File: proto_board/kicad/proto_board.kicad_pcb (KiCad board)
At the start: 2 copper layers, 80 x 50 mm, 3 parts, among them J1 pcie_98

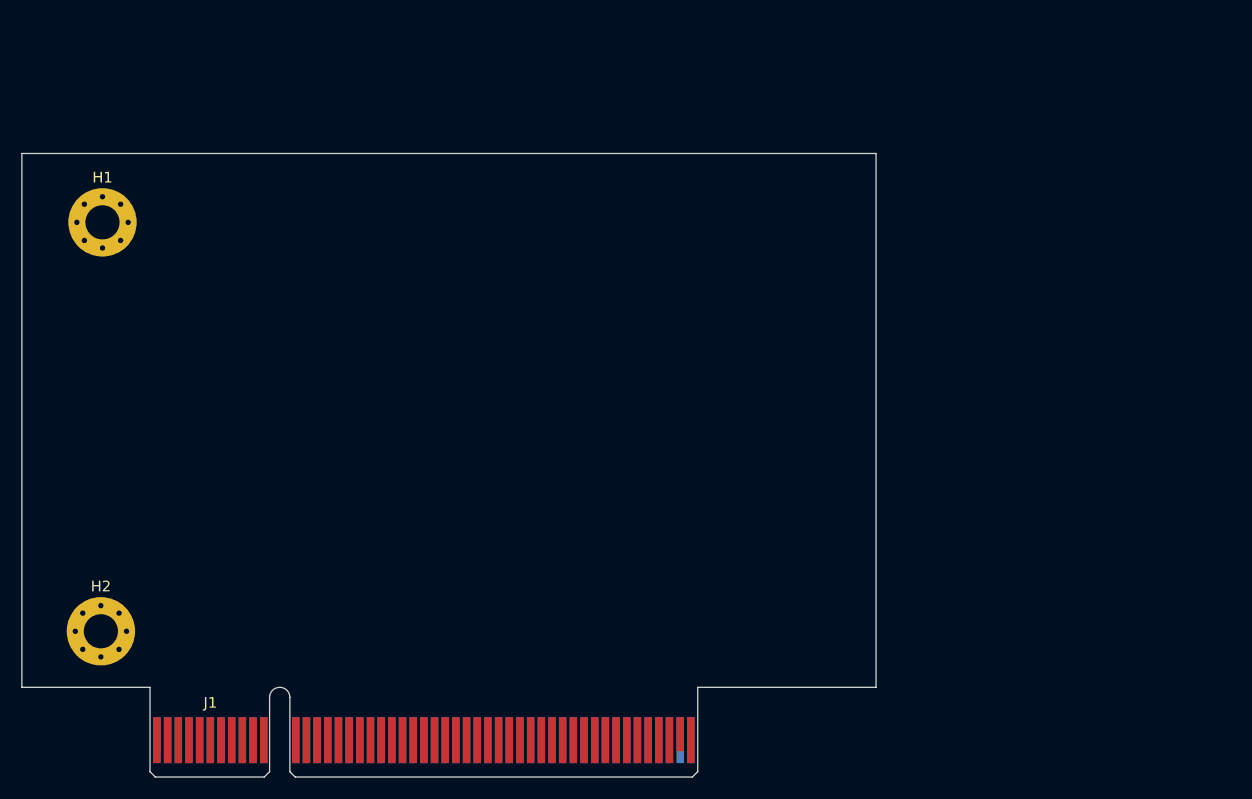
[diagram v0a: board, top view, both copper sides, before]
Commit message: Proto board work in progress.
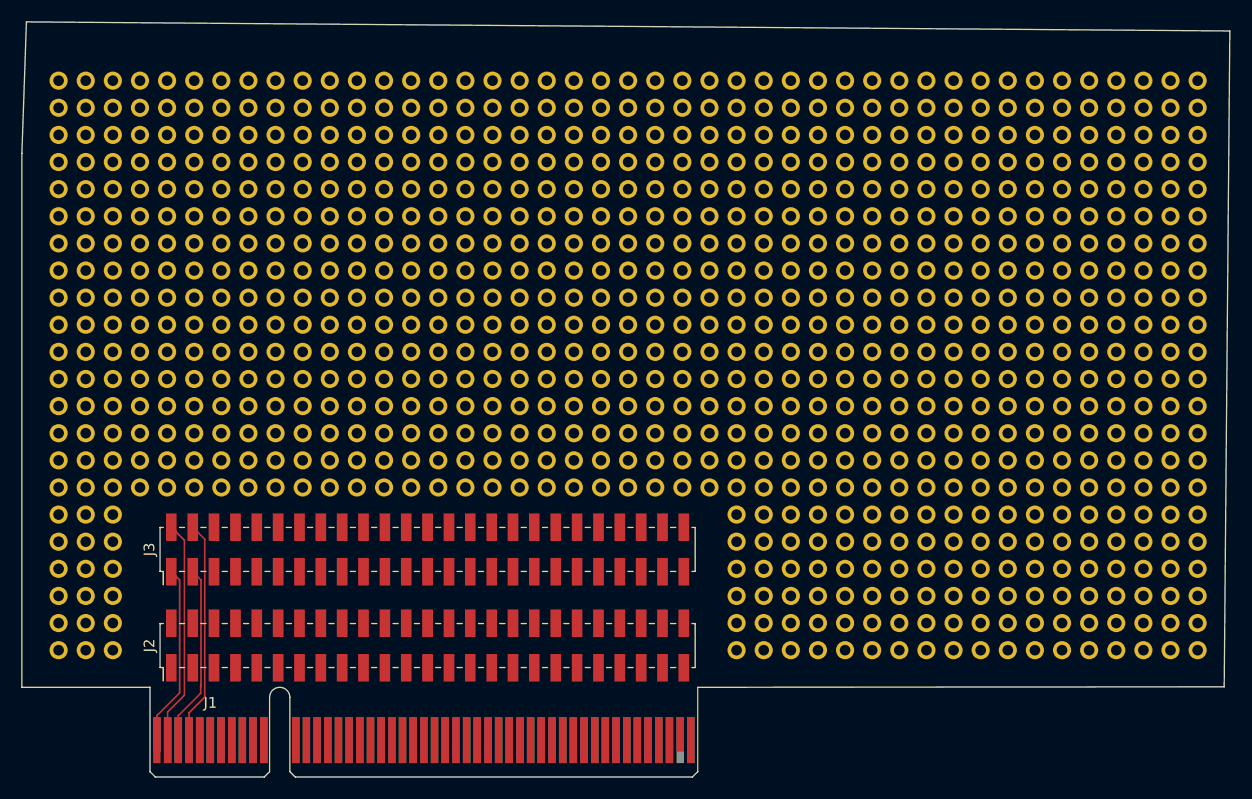
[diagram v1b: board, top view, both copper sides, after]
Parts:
- removed H1, H2: Bracket Hole, MountingHole:MountingHole_3.2mm_M3_Pad_Via
- added J2: Conn_02x25_Odd_Even, Connector_PinHeader_2.00mm:PinHeader_2x25_P2.00mm_Vertical_SMD, F.Cu at (126.0, 96.1)
- added J3: Conn_02x25_Odd_Even, Connector_PinHeader_2.00mm:PinHeader_2x25_P2.00mm_Vertical_SMD, F.Cu at (126.0, 87.1)
- added TP1: TestPoint, proto_board:pad, F.Cu at (147.3, 55.9)
- added TP1: TestPoint, proto_board:pad, F.Cu at (144.8, 55.9)
- added TP1: TestPoint, proto_board:pad, F.Cu at (162.6, 86.4)
- added TP1: TestPoint, proto_board:pad, F.Cu at (149.9, 78.7)
- added TP1: TestPoint, proto_board:pad, F.Cu at (94.0, 58.4)
- added TP1: TestPoint, proto_board:pad, F.Cu at (129.5, 53.3)
- added TP1: TestPoint, proto_board:pad, F.Cu at (175.3, 86.4)
- added TP1: TestPoint, proto_board:pad, F.Cu at (157.5, 83.8)
- added TP1: TestPoint, proto_board:pad, F.Cu at (177.8, 43.2)
- added TP1: TestPoint, proto_board:pad, F.Cu at (170.2, 78.7)
- added TP1: TestPoint, proto_board:pad, F.Cu at (144.8, 81.3)
- added TP1: TestPoint, proto_board:pad, F.Cu at (142.2, 50.8)
- added TP1: TestPoint, proto_board:pad, F.Cu at (190.5, 43.2)
- added TP1: TestPoint, proto_board:pad, F.Cu at (127.0, 43.2)
- added TP1: TestPoint, proto_board:pad, F.Cu at (134.6, 50.8)
- added TP1: TestPoint, proto_board:pad, F.Cu at (114.3, 73.7)
- added TP1: TestPoint, proto_board:pad, F.Cu at (167.6, 66.0)
- added TP1: TestPoint, proto_board:pad, F.Cu at (180.3, 53.3)
- added TP1: TestPoint, proto_board:pad, F.Cu at (94.0, 76.2)
- added TP1: TestPoint, proto_board:pad, F.Cu at (175.3, 81.3)
- added TP1: TestPoint, proto_board:pad, F.Cu at (165.1, 91.4)
- added TP1: TestPoint, proto_board:pad, F.Cu at (101.6, 71.1)
- added TP1: TestPoint, proto_board:pad, F.Cu at (185.4, 81.3)
- added TP1: TestPoint, proto_board:pad, F.Cu at (101.6, 73.7)
- added TP1: TestPoint, proto_board:pad, F.Cu at (188.0, 81.3)
- added TP1: TestPoint, proto_board:pad, F.Cu at (180.3, 83.8)
- added TP1: TestPoint, proto_board:pad, F.Cu at (165.1, 81.3)
- added TP1: TestPoint, proto_board:pad, F.Cu at (188.0, 73.7)
- added TP1: TestPoint, proto_board:pad, F.Cu at (195.6, 83.8)
- added TP1: TestPoint, proto_board:pad, F.Cu at (111.8, 78.7)
- added TP1: TestPoint, proto_board:pad, F.Cu at (127.0, 73.7)
- added TP1: TestPoint, proto_board:pad, F.Cu at (139.7, 61.0)
- added TP1: TestPoint, proto_board:pad, F.Cu at (185.4, 61.0)
- added TP1: TestPoint, proto_board:pad, F.Cu at (180.3, 81.3)
- added TP1: TestPoint, proto_board:pad, F.Cu at (101.6, 76.2)
- added TP1: TestPoint, proto_board:pad, F.Cu at (170.2, 61.0)
- added TP1: TestPoint, proto_board:pad, F.Cu at (101.6, 43.2)
- added TP1: TestPoint, proto_board:pad, F.Cu at (144.8, 66.0)
- added TP1: TestPoint, proto_board:pad, F.Cu at (175.3, 45.7)
- added TP1: TestPoint, proto_board:pad, F.Cu at (96.5, 88.9)
- added TP1: TestPoint, proto_board:pad, F.Cu at (152.4, 68.6)
- added TP1: TestPoint, proto_board:pad, F.Cu at (180.3, 91.4)
- added TP1: TestPoint, proto_board:pad, F.Cu at (91.4, 68.6)
- added TP1: TestPoint, proto_board:pad, F.Cu at (134.6, 48.3)
- added TP1: TestPoint, proto_board:pad, F.Cu at (170.2, 68.6)
- added TP1: TestPoint, proto_board:pad, F.Cu at (142.2, 55.9)
- added TP1: TestPoint, proto_board:pad, F.Cu at (167.6, 96.5)
- added TP1: TestPoint, proto_board:pad, F.Cu at (94.0, 63.5)
- added TP1: TestPoint, proto_board:pad, F.Cu at (96.5, 53.3)
- added TP1: TestPoint, proto_board:pad, F.Cu at (144.8, 48.3)
- added TP1: TestPoint, proto_board:pad, F.Cu at (124.5, 50.8)
- added TP1: TestPoint, proto_board:pad, F.Cu at (111.8, 43.2)
- added TP1: TestPoint, proto_board:pad, F.Cu at (91.4, 61.0)
- added TP1: TestPoint, proto_board:pad, F.Cu at (149.9, 48.3)
- added TP1: TestPoint, proto_board:pad, F.Cu at (106.7, 50.8)
- added TP1: TestPoint, proto_board:pad, F.Cu at (132.1, 76.2)
- added TP1: TestPoint, proto_board:pad, F.Cu at (114.3, 71.1)
- added TP1: TestPoint, proto_board:pad, F.Cu at (177.8, 76.2)
- added TP1: TestPoint, proto_board:pad, F.Cu at (94.0, 68.6)
- added TP1: TestPoint, proto_board:pad, F.Cu at (137.2, 66.0)
- added TP1: TestPoint, proto_board:pad, F.Cu at (195.6, 86.4)
- added TP1: TestPoint, proto_board:pad, F.Cu at (185.4, 78.7)
- added TP1: TestPoint, proto_board:pad, F.Cu at (152.4, 55.9)
- added TP1: TestPoint, proto_board:pad, F.Cu at (193.0, 48.3)
- added TP1: TestPoint, proto_board:pad, F.Cu at (198.1, 73.7)
- added TP1: TestPoint, proto_board:pad, F.Cu at (160.0, 96.5)
- added TP1: TestPoint, proto_board:pad, F.Cu at (129.5, 68.6)
- added TP1: TestPoint, proto_board:pad, F.Cu at (180.3, 58.4)
- added TP1: TestPoint, proto_board:pad, F.Cu at (190.5, 96.5)
- added TP1: TestPoint, proto_board:pad, F.Cu at (121.9, 50.8)
- added TP1: TestPoint, proto_board:pad, F.Cu at (142.2, 43.2)
- added TP1: TestPoint, proto_board:pad, F.Cu at (132.1, 50.8)
- added TP1: TestPoint, proto_board:pad, F.Cu at (182.9, 58.4)
- added TP1: TestPoint, proto_board:pad, F.Cu at (195.6, 96.5)
- added TP1: TestPoint, proto_board:pad, F.Cu at (177.8, 58.4)
- added TP1: TestPoint, proto_board:pad, F.Cu at (99.1, 73.7)
- added TP1: TestPoint, proto_board:pad, F.Cu at (167.6, 45.7)
- added TP1: TestPoint, proto_board:pad, F.Cu at (190.5, 55.9)
- added TP1: TestPoint, proto_board:pad, F.Cu at (137.2, 71.1)
- added TP1: TestPoint, proto_board:pad, F.Cu at (147.3, 58.4)
- added TP1: TestPoint, proto_board:pad, F.Cu at (177.8, 83.8)
- added TP1: TestPoint, proto_board:pad, F.Cu at (139.7, 55.9)
- added TP1: TestPoint, proto_board:pad, F.Cu at (165.1, 66.0)
- added TP1: TestPoint, proto_board:pad, F.Cu at (154.9, 96.5)
- added TP1: TestPoint, proto_board:pad, F.Cu at (172.7, 94.0)
- added TP1: TestPoint, proto_board:pad, F.Cu at (152.4, 50.8)
- added TP1: TestPoint, proto_board:pad, F.Cu at (127.0, 53.3)
- added TP1: TestPoint, proto_board:pad, F.Cu at (139.7, 76.2)
- added TP1: TestPoint, proto_board:pad, F.Cu at (96.5, 50.8)
- added TP1: TestPoint, proto_board:pad, F.Cu at (195.6, 94.0)
- added TP1: TestPoint, proto_board:pad, F.Cu at (106.7, 66.0)
- added TP1: TestPoint, proto_board:pad, F.Cu at (198.1, 63.5)
- added TP1: TestPoint, proto_board:pad, F.Cu at (99.1, 58.4)
- added TP1: TestPoint, proto_board:pad, F.Cu at (99.1, 76.2)
- added TP1: TestPoint, proto_board:pad, F.Cu at (106.7, 61.0)
- added TP1: TestPoint, proto_board:pad, F.Cu at (167.6, 76.2)
- added TP1: TestPoint, proto_board:pad, F.Cu at (91.4, 50.8)
- added TP1: TestPoint, proto_board:pad, F.Cu at (185.4, 71.1)
- added TP1: TestPoint, proto_board:pad, F.Cu at (193.0, 96.5)
- added TP1: TestPoint, proto_board:pad, F.Cu at (193.0, 94.0)
- added TP1: TestPoint, proto_board:pad, F.Cu at (129.5, 61.0)
- added TP1: TestPoint, proto_board:pad, F.Cu at (124.5, 71.1)
- added TP1: TestPoint, proto_board:pad, F.Cu at (129.5, 58.4)
- added TP1: TestPoint, proto_board:pad, F.Cu at (144.8, 76.2)
- added TP1: TestPoint, proto_board:pad, F.Cu at (96.5, 58.4)
- added TP1: TestPoint, proto_board:pad, F.Cu at (188.0, 45.7)
- added TP1: TestPoint, proto_board:pad, F.Cu at (139.7, 50.8)
- added TP1: TestPoint, proto_board:pad, F.Cu at (114.3, 61.0)
- added TP1: TestPoint, proto_board:pad, F.Cu at (188.0, 96.5)
- added TP1: TestPoint, proto_board:pad, F.Cu at (198.1, 43.2)
- added TP1: TestPoint, proto_board:pad, F.Cu at (185.4, 53.3)
- added TP1: TestPoint, proto_board:pad, F.Cu at (96.5, 63.5)
- added TP1: TestPoint, proto_board:pad, F.Cu at (195.6, 68.6)
- added TP1: TestPoint, proto_board:pad, F.Cu at (182.9, 96.5)
- added TP1: TestPoint, proto_board:pad, F.Cu at (180.3, 61.0)
- added TP1: TestPoint, proto_board:pad, F.Cu at (129.5, 48.3)
- added TP1: TestPoint, proto_board:pad, F.Cu at (160.0, 94.0)
- added TP1: TestPoint, proto_board:pad, F.Cu at (188.0, 68.6)
- added TP1: TestPoint, proto_board:pad, F.Cu at (170.2, 55.9)
- added TP1: TestPoint, proto_board:pad, F.Cu at (185.4, 91.4)
- added TP1: TestPoint, proto_board:pad, F.Cu at (180.3, 86.4)
- added TP1: TestPoint, proto_board:pad, F.Cu at (160.0, 61.0)
- added TP1: TestPoint, proto_board:pad, F.Cu at (185.4, 63.5)
- added TP1: TestPoint, proto_board:pad, F.Cu at (195.6, 55.9)
- added TP1: TestPoint, proto_board:pad, F.Cu at (182.9, 83.8)
- added TP1: TestPoint, proto_board:pad, F.Cu at (162.6, 76.2)
- added TP1: TestPoint, proto_board:pad, F.Cu at (154.9, 91.4)
- added TP1: TestPoint, proto_board:pad, F.Cu at (154.9, 45.7)
- added TP1: TestPoint, proto_board:pad, F.Cu at (162.6, 58.4)
- added TP1: TestPoint, proto_board:pad, F.Cu at (147.3, 53.3)
- added TP1: TestPoint, proto_board:pad, F.Cu at (124.5, 66.0)
- added TP1: TestPoint, proto_board:pad, F.Cu at (149.9, 76.2)
- added TP1: TestPoint, proto_board:pad, F.Cu at (170.2, 96.5)
- added TP1: TestPoint, proto_board:pad, F.Cu at (172.7, 50.8)
- added TP1: TestPoint, proto_board:pad, F.Cu at (94.0, 48.3)
- added TP1: TestPoint, proto_board:pad, F.Cu at (177.8, 86.4)
- added TP1: TestPoint, proto_board:pad, F.Cu at (149.9, 66.0)
- added TP1: TestPoint, proto_board:pad, F.Cu at (127.0, 58.4)
- added TP1: TestPoint, proto_board:pad, F.Cu at (119.4, 50.8)
- added TP1: TestPoint, proto_board:pad, F.Cu at (124.5, 45.7)
- added TP1: TestPoint, proto_board:pad, F.Cu at (190.5, 68.6)
- added TP1: TestPoint, proto_board:pad, F.Cu at (137.2, 73.7)
- added TP1: TestPoint, proto_board:pad, F.Cu at (193.0, 86.4)
- added TP1: TestPoint, proto_board:pad, F.Cu at (157.5, 53.3)
- added TP1: TestPoint, proto_board:pad, F.Cu at (165.1, 68.6)
- added TP1: TestPoint, proto_board:pad, F.Cu at (167.6, 81.3)
- added TP1: TestPoint, proto_board:pad, F.Cu at (198.1, 91.4)
- added TP1: TestPoint, proto_board:pad, F.Cu at (162.6, 50.8)
- added TP1: TestPoint, proto_board:pad, F.Cu at (147.3, 63.5)
- added TP1: TestPoint, proto_board:pad, F.Cu at (198.1, 88.9)
- added TP1: TestPoint, proto_board:pad, F.Cu at (154.9, 73.7)
- added TP1: TestPoint, proto_board:pad, F.Cu at (182.9, 55.9)
- added TP1: TestPoint, proto_board:pad, F.Cu at (162.6, 91.4)
- added TP1: TestPoint, proto_board:pad, F.Cu at (109.2, 71.1)
- added TP1: TestPoint, proto_board:pad, F.Cu at (167.6, 94.0)
- added TP1: TestPoint, proto_board:pad, F.Cu at (188.0, 66.0)
- added TP1: TestPoint, proto_board:pad, F.Cu at (129.5, 81.3)
- added TP1: TestPoint, proto_board:pad, F.Cu at (109.2, 50.8)
- added TP1: TestPoint, proto_board:pad, F.Cu at (198.1, 61.0)
- added TP1: TestPoint, proto_board:pad, F.Cu at (182.9, 78.7)
- added TP1: TestPoint, proto_board:pad, F.Cu at (144.8, 50.8)
- added TP1: TestPoint, proto_board:pad, F.Cu at (147.3, 50.8)
- added TP1: TestPoint, proto_board:pad, F.Cu at (104.1, 68.6)
- added TP1: TestPoint, proto_board:pad, F.Cu at (195.6, 53.3)
- added TP1: TestPoint, proto_board:pad, F.Cu at (101.6, 63.5)
- added TP1: TestPoint, proto_board:pad, F.Cu at (111.8, 48.3)
- added TP1: TestPoint, proto_board:pad, F.Cu at (167.6, 63.5)
- added TP1: TestPoint, proto_board:pad, F.Cu at (142.2, 53.3)
- added TP1: TestPoint, proto_board:pad, F.Cu at (134.6, 45.7)
- added TP1: TestPoint, proto_board:pad, F.Cu at (109.2, 63.5)
- added TP1: TestPoint, proto_board:pad, F.Cu at (124.5, 81.3)
- added TP1: TestPoint, proto_board:pad, F.Cu at (162.6, 81.3)
- added TP1: TestPoint, proto_board:pad, F.Cu at (134.6, 81.3)
- added TP1: TestPoint, proto_board:pad, F.Cu at (137.2, 58.4)
- added TP1: TestPoint, proto_board:pad, F.Cu at (154.9, 88.9)
- added TP1: TestPoint, proto_board:pad, F.Cu at (152.4, 48.3)
- added TP1: TestPoint, proto_board:pad, F.Cu at (172.7, 96.5)
- added TP1: TestPoint, proto_board:pad, F.Cu at (94.0, 83.8)
- added TP1: TestPoint, proto_board:pad, F.Cu at (175.3, 55.9)
- added TP1: TestPoint, proto_board:pad, F.Cu at (119.4, 55.9)
- added TP1: TestPoint, proto_board:pad, F.Cu at (162.6, 66.0)
- added TP1: TestPoint, proto_board:pad, F.Cu at (142.2, 73.7)
- added TP1: TestPoint, proto_board:pad, F.Cu at (198.1, 96.5)
- added TP1: TestPoint, proto_board:pad, F.Cu at (152.4, 45.7)
- added TP1: TestPoint, proto_board:pad, F.Cu at (121.9, 55.9)
- added TP1: TestPoint, proto_board:pad, F.Cu at (195.6, 63.5)
- added TP1: TestPoint, proto_board:pad, F.Cu at (111.8, 71.1)
- added TP1: TestPoint, proto_board:pad, F.Cu at (157.5, 94.0)
- added TP1: TestPoint, proto_board:pad, F.Cu at (188.0, 71.1)
- added TP1: TestPoint, proto_board:pad, F.Cu at (170.2, 88.9)
- added TP1: TestPoint, proto_board:pad, F.Cu at (119.4, 43.2)
- added TP1: TestPoint, proto_board:pad, F.Cu at (111.8, 61.0)
- added TP1: TestPoint, proto_board:pad, F.Cu at (147.3, 78.7)
- added TP1: TestPoint, proto_board:pad, F.Cu at (154.9, 66.0)
- added TP1: TestPoint, proto_board:pad, F.Cu at (106.7, 78.7)
- added TP1: TestPoint, proto_board:pad, F.Cu at (172.7, 53.3)
- added TP1: TestPoint, proto_board:pad, F.Cu at (182.9, 76.2)
- added TP1: TestPoint, proto_board:pad, F.Cu at (147.3, 71.1)
- added TP1: TestPoint, proto_board:pad, F.Cu at (157.5, 76.2)
- added TP1: TestPoint, proto_board:pad, F.Cu at (109.2, 66.0)
- added TP1: TestPoint, proto_board:pad, F.Cu at (114.3, 58.4)
- added TP1: TestPoint, proto_board:pad, F.Cu at (185.4, 66.0)
- added TP1: TestPoint, proto_board:pad, F.Cu at (195.6, 66.0)
- added TP1: TestPoint, proto_board:pad, F.Cu at (99.1, 68.6)
- added TP1: TestPoint, proto_board:pad, F.Cu at (127.0, 55.9)
- added TP1: TestPoint, proto_board:pad, F.Cu at (121.9, 63.5)
- added TP1: TestPoint, proto_board:pad, F.Cu at (121.9, 78.7)
- added TP1: TestPoint, proto_board:pad, F.Cu at (144.8, 43.2)
- added TP1: TestPoint, proto_board:pad, F.Cu at (116.8, 78.7)
- added TP1: TestPoint, proto_board:pad, F.Cu at (119.4, 53.3)
- added TP1: TestPoint, proto_board:pad, F.Cu at (124.5, 58.4)
- added TP1: TestPoint, proto_board:pad, F.Cu at (149.9, 81.3)
- added TP1: TestPoint, proto_board:pad, F.Cu at (190.5, 88.9)
- added TP1: TestPoint, proto_board:pad, F.Cu at (175.3, 88.9)
- added TP1: TestPoint, proto_board:pad, F.Cu at (182.9, 50.8)
- added TP1: TestPoint, proto_board:pad, F.Cu at (111.8, 76.2)
- added TP1: TestPoint, proto_board:pad, F.Cu at (165.1, 73.7)
- added TP1: TestPoint, proto_board:pad, F.Cu at (96.5, 76.2)
- added TP1: TestPoint, proto_board:pad, F.Cu at (162.6, 78.7)
- added TP1: TestPoint, proto_board:pad, F.Cu at (147.3, 73.7)
- added TP1: TestPoint, proto_board:pad, F.Cu at (170.2, 86.4)
- added TP1: TestPoint, proto_board:pad, F.Cu at (121.9, 76.2)
- added TP1: TestPoint, proto_board:pad, F.Cu at (193.0, 81.3)
- added TP1: TestPoint, proto_board:pad, F.Cu at (142.2, 78.7)
- added TP1: TestPoint, proto_board:pad, F.Cu at (182.9, 94.0)
- added TP1: TestPoint, proto_board:pad, F.Cu at (91.4, 76.2)
- added TP1: TestPoint, proto_board:pad, F.Cu at (139.7, 53.3)
- added TP1: TestPoint, proto_board:pad, F.Cu at (188.0, 55.9)
- added TP1: TestPoint, proto_board:pad, F.Cu at (175.3, 76.2)
- added TP1: TestPoint, proto_board:pad, F.Cu at (193.0, 91.4)
- added TP1: TestPoint, proto_board:pad, F.Cu at (106.7, 45.7)
- added TP1: TestPoint, proto_board:pad, F.Cu at (170.2, 76.2)
- added TP1: TestPoint, proto_board:pad, F.Cu at (127.0, 81.3)
- added TP1: TestPoint, proto_board:pad, F.Cu at (188.0, 61.0)
- added TP1: TestPoint, proto_board:pad, F.Cu at (160.0, 76.2)
- added TP1: TestPoint, proto_board:pad, F.Cu at (109.2, 55.9)
- added TP1: TestPoint, proto_board:pad, F.Cu at (94.0, 50.8)
- added TP1: TestPoint, proto_board:pad, F.Cu at (111.8, 81.3)
- added TP1: TestPoint, proto_board:pad, F.Cu at (190.5, 58.4)
- added TP1: TestPoint, proto_board:pad, F.Cu at (116.8, 48.3)
- added TP1: TestPoint, proto_board:pad, F.Cu at (109.2, 48.3)
- added TP1: TestPoint, proto_board:pad, F.Cu at (152.4, 81.3)
- added TP1: TestPoint, proto_board:pad, F.Cu at (157.5, 73.7)
- added TP1: TestPoint, proto_board:pad, F.Cu at (195.6, 48.3)
- added TP1: TestPoint, proto_board:pad, F.Cu at (170.2, 58.4)
- added TP1: TestPoint, proto_board:pad, F.Cu at (165.1, 45.7)
- added TP1: TestPoint, proto_board:pad, F.Cu at (177.8, 45.7)
- added TP1: TestPoint, proto_board:pad, F.Cu at (137.2, 68.6)
- added TP1: TestPoint, proto_board:pad, F.Cu at (127.0, 78.7)
- added TP1: TestPoint, proto_board:pad, F.Cu at (129.5, 71.1)
- added TP1: TestPoint, proto_board:pad, F.Cu at (198.1, 81.3)
- added TP1: TestPoint, proto_board:pad, F.Cu at (175.3, 58.4)
- added TP1: TestPoint, proto_board:pad, F.Cu at (182.9, 81.3)
- added TP1: TestPoint, proto_board:pad, F.Cu at (170.2, 83.8)
- added TP1: TestPoint, proto_board:pad, F.Cu at (129.5, 55.9)
- added TP1: TestPoint, proto_board:pad, F.Cu at (165.1, 61.0)
- added TP1: TestPoint, proto_board:pad, F.Cu at (124.5, 43.2)
- added TP1: TestPoint, proto_board:pad, F.Cu at (139.7, 78.7)
- added TP1: TestPoint, proto_board:pad, F.Cu at (172.7, 68.6)
- added TP1: TestPoint, proto_board:pad, F.Cu at (172.7, 76.2)
- added TP1: TestPoint, proto_board:pad, F.Cu at (132.1, 48.3)
- added TP1: TestPoint, proto_board:pad, F.Cu at (127.0, 48.3)
- added TP1: TestPoint, proto_board:pad, F.Cu at (132.1, 66.0)
- added TP1: TestPoint, proto_board:pad, F.Cu at (157.5, 86.4)
- added TP1: TestPoint, proto_board:pad, F.Cu at (157.5, 48.3)
- added TP1: TestPoint, proto_board:pad, F.Cu at (175.3, 43.2)
- added TP1: TestPoint, proto_board:pad, F.Cu at (185.4, 50.8)
- added TP1: TestPoint, proto_board:pad, F.Cu at (96.5, 73.7)
- added TP1: TestPoint, proto_board:pad, F.Cu at (147.3, 61.0)
- added TP1: TestPoint, proto_board:pad, F.Cu at (116.8, 50.8)
- added TP1: TestPoint, proto_board:pad, F.Cu at (154.9, 53.3)
- added TP1: TestPoint, proto_board:pad, F.Cu at (154.9, 94.0)
- added TP1: TestPoint, proto_board:pad, F.Cu at (157.5, 55.9)
- added TP1: TestPoint, proto_board:pad, F.Cu at (116.8, 76.2)
- added TP1: TestPoint, proto_board:pad, F.Cu at (139.7, 66.0)
- added TP1: TestPoint, proto_board:pad, F.Cu at (142.2, 45.7)
- added TP1: TestPoint, proto_board:pad, F.Cu at (182.9, 43.2)
- added TP1: TestPoint, proto_board:pad, F.Cu at (96.5, 83.8)
- added TP1: TestPoint, proto_board:pad, F.Cu at (119.4, 81.3)
- added TP1: TestPoint, proto_board:pad, F.Cu at (94.0, 66.0)
- added TP1: TestPoint, proto_board:pad, F.Cu at (188.0, 63.5)
- added TP1: TestPoint, proto_board:pad, F.Cu at (111.8, 68.6)
- added TP1: TestPoint, proto_board:pad, F.Cu at (157.5, 91.4)
- added TP1: TestPoint, proto_board:pad, F.Cu at (175.3, 53.3)
- added TP1: TestPoint, proto_board:pad, F.Cu at (106.7, 53.3)
- added TP1: TestPoint, proto_board:pad, F.Cu at (119.4, 68.6)
- added TP1: TestPoint, proto_board:pad, F.Cu at (180.3, 88.9)
- added TP1: TestPoint, proto_board:pad, F.Cu at (142.2, 58.4)
- added TP1: TestPoint, proto_board:pad, F.Cu at (94.0, 78.7)
- added TP1: TestPoint, proto_board:pad, F.Cu at (157.5, 58.4)
- added TP1: TestPoint, proto_board:pad, F.Cu at (139.7, 43.2)
- added TP1: TestPoint, proto_board:pad, F.Cu at (182.9, 45.7)
- added TP1: TestPoint, proto_board:pad, F.Cu at (177.8, 91.4)
- added TP1: TestPoint, proto_board:pad, F.Cu at (152.4, 76.2)
- added TP1: TestPoint, proto_board:pad, F.Cu at (96.5, 61.0)
- added TP1: TestPoint, proto_board:pad, F.Cu at (180.3, 63.5)
- added TP1: TestPoint, proto_board:pad, F.Cu at (149.9, 61.0)
- added TP1: TestPoint, proto_board:pad, F.Cu at (195.6, 81.3)
- added TP1: TestPoint, proto_board:pad, F.Cu at (106.7, 63.5)
- added TP1: TestPoint, proto_board:pad, F.Cu at (137.2, 48.3)
- added TP1: TestPoint, proto_board:pad, F.Cu at (165.1, 76.2)
- added TP1: TestPoint, proto_board:pad, F.Cu at (91.4, 55.9)
- added TP1: TestPoint, proto_board:pad, F.Cu at (157.5, 71.1)
- added TP1: TestPoint, proto_board:pad, F.Cu at (137.2, 61.0)
- added TP1: TestPoint, proto_board:pad, F.Cu at (193.0, 53.3)
- added TP1: TestPoint, proto_board:pad, F.Cu at (190.5, 71.1)
- added TP1: TestPoint, proto_board:pad, F.Cu at (172.7, 61.0)
- added TP1: TestPoint, proto_board:pad, F.Cu at (157.5, 68.6)
- added TP1: TestPoint, proto_board:pad, F.Cu at (127.0, 63.5)
- added TP1: TestPoint, proto_board:pad, F.Cu at (119.4, 73.7)
- added TP1: TestPoint, proto_board:pad, F.Cu at (160.0, 68.6)
- added TP1: TestPoint, proto_board:pad, F.Cu at (160.0, 81.3)
- added TP1: TestPoint, proto_board:pad, F.Cu at (172.7, 43.2)
- added TP1: TestPoint, proto_board:pad, F.Cu at (94.0, 96.5)
- added TP1: TestPoint, proto_board:pad, F.Cu at (104.1, 45.7)
- added TP1: TestPoint, proto_board:pad, F.Cu at (152.4, 43.2)
- added TP1: TestPoint, proto_board:pad, F.Cu at (170.2, 43.2)
- added TP1: TestPoint, proto_board:pad, F.Cu at (190.5, 94.0)
- added TP1: TestPoint, proto_board:pad, F.Cu at (198.1, 68.6)
- added TP1: TestPoint, proto_board:pad, F.Cu at (195.6, 88.9)
- added TP1: TestPoint, proto_board:pad, F.Cu at (154.9, 81.3)
- added TP1: TestPoint, proto_board:pad, F.Cu at (99.1, 66.0)
- added TP1: TestPoint, proto_board:pad, F.Cu at (144.8, 45.7)
- added TP1: TestPoint, proto_board:pad, F.Cu at (157.5, 96.5)
- added TP1: TestPoint, proto_board:pad, F.Cu at (124.5, 48.3)
- added TP1: TestPoint, proto_board:pad, F.Cu at (101.6, 81.3)
- added TP1: TestPoint, proto_board:pad, F.Cu at (175.3, 50.8)
- added TP1: TestPoint, proto_board:pad, F.Cu at (139.7, 58.4)
- added TP1: TestPoint, proto_board:pad, F.Cu at (160.0, 66.0)
- added TP1: TestPoint, proto_board:pad, F.Cu at (157.5, 88.9)
- added TP1: TestPoint, proto_board:pad, F.Cu at (154.9, 83.8)
- added TP1: TestPoint, proto_board:pad, F.Cu at (147.3, 43.2)
- added TP1: TestPoint, proto_board:pad, F.Cu at (101.6, 58.4)
- added TP1: TestPoint, proto_board:pad, F.Cu at (139.7, 71.1)
- added TP1: TestPoint, proto_board:pad, F.Cu at (172.7, 71.1)
- added TP1: TestPoint, proto_board:pad, F.Cu at (160.0, 91.4)
- added TP1: TestPoint, proto_board:pad, F.Cu at (172.7, 45.7)
- added TP1: TestPoint, proto_board:pad, F.Cu at (137.2, 81.3)
- added TP1: TestPoint, proto_board:pad, F.Cu at (188.0, 76.2)
- added TP1: TestPoint, proto_board:pad, F.Cu at (170.2, 66.0)
- added TP1: TestPoint, proto_board:pad, F.Cu at (190.5, 81.3)
- added TP1: TestPoint, proto_board:pad, F.Cu at (182.9, 48.3)
- added TP1: TestPoint, proto_board:pad, F.Cu at (185.4, 73.7)
- added TP1: TestPoint, proto_board:pad, F.Cu at (137.2, 53.3)
- added TP1: TestPoint, proto_board:pad, F.Cu at (160.0, 73.7)
- added TP1: TestPoint, proto_board:pad, F.Cu at (172.7, 55.9)
- added TP1: TestPoint, proto_board:pad, F.Cu at (162.6, 83.8)
- added TP1: TestPoint, proto_board:pad, F.Cu at (104.1, 50.8)
- added TP1: TestPoint, proto_board:pad, F.Cu at (172.7, 63.5)
- added TP1: TestPoint, proto_board:pad, F.Cu at (121.9, 68.6)
- added TP1: TestPoint, proto_board:pad, F.Cu at (193.0, 66.0)
- added TP1: TestPoint, proto_board:pad, F.Cu at (175.3, 73.7)
- added TP1: TestPoint, proto_board:pad, F.Cu at (96.5, 94.0)
- added TP1: TestPoint, proto_board:pad, F.Cu at (91.4, 58.4)
- added TP1: TestPoint, proto_board:pad, F.Cu at (185.4, 76.2)
- added TP1: TestPoint, proto_board:pad, F.Cu at (185.4, 68.6)
- added TP1: TestPoint, proto_board:pad, F.Cu at (193.0, 58.4)
- added TP1: TestPoint, proto_board:pad, F.Cu at (147.3, 68.6)
- added TP1: TestPoint, proto_board:pad, F.Cu at (96.5, 78.7)
- added TP1: TestPoint, proto_board:pad, F.Cu at (170.2, 91.4)
- added TP1: TestPoint, proto_board:pad, F.Cu at (134.6, 63.5)
- added TP1: TestPoint, proto_board:pad, F.Cu at (134.6, 55.9)
- added TP1: TestPoint, proto_board:pad, F.Cu at (99.1, 53.3)
- added TP1: TestPoint, proto_board:pad, F.Cu at (124.5, 53.3)
- added TP1: TestPoint, proto_board:pad, F.Cu at (104.1, 81.3)
- added TP1: TestPoint, proto_board:pad, F.Cu at (193.0, 55.9)
- added TP1: TestPoint, proto_board:pad, F.Cu at (91.4, 78.7)
- added TP1: TestPoint, proto_board:pad, F.Cu at (172.7, 73.7)
- added TP1: TestPoint, proto_board:pad, F.Cu at (152.4, 73.7)
- added TP1: TestPoint, proto_board:pad, F.Cu at (193.0, 50.8)
- added TP1: TestPoint, proto_board:pad, F.Cu at (190.5, 48.3)
- added TP1: TestPoint, proto_board:pad, F.Cu at (182.9, 63.5)
- added TP1: TestPoint, proto_board:pad, F.Cu at (142.2, 48.3)
- added TP1: TestPoint, proto_board:pad, F.Cu at (172.7, 88.9)
- added TP1: TestPoint, proto_board:pad, F.Cu at (121.9, 45.7)
- added TP1: TestPoint, proto_board:pad, F.Cu at (137.2, 78.7)
- added TP1: TestPoint, proto_board:pad, F.Cu at (185.4, 96.5)
- added TP1: TestPoint, proto_board:pad, F.Cu at (195.6, 45.7)
- added TP1: TestPoint, proto_board:pad, F.Cu at (109.2, 76.2)
- added TP1: TestPoint, proto_board:pad, F.Cu at (142.2, 68.6)
- added TP1: TestPoint, proto_board:pad, F.Cu at (119.4, 58.4)
- added TP1: TestPoint, proto_board:pad, F.Cu at (137.2, 45.7)
- added TP1: TestPoint, proto_board:pad, F.Cu at (170.2, 73.7)
- added TP1: TestPoint, proto_board:pad, F.Cu at (91.4, 63.5)
- added TP1: TestPoint, proto_board:pad, F.Cu at (111.8, 73.7)
- added TP1: TestPoint, proto_board:pad, F.Cu at (109.2, 53.3)
- added TP1: TestPoint, proto_board:pad, F.Cu at (129.5, 50.8)
- added TP1: TestPoint, proto_board:pad, F.Cu at (165.1, 58.4)
- added TP1: TestPoint, proto_board:pad, F.Cu at (132.1, 78.7)
- added TP1: TestPoint, proto_board:pad, F.Cu at (160.0, 78.7)
- added TP1: TestPoint, proto_board:pad, F.Cu at (121.9, 71.1)
- added TP1: TestPoint, proto_board:pad, F.Cu at (139.7, 68.6)
- added TP1: TestPoint, proto_board:pad, F.Cu at (91.4, 48.3)
- added TP1: TestPoint, proto_board:pad, F.Cu at (101.6, 68.6)
- added TP1: TestPoint, proto_board:pad, F.Cu at (165.1, 83.8)
- added TP1: TestPoint, proto_board:pad, F.Cu at (175.3, 66.0)
- added TP1: TestPoint, proto_board:pad, F.Cu at (154.9, 71.1)
- added TP1: TestPoint, proto_board:pad, F.Cu at (188.0, 86.4)
- added TP1: TestPoint, proto_board:pad, F.Cu at (104.1, 61.0)
- added TP1: TestPoint, proto_board:pad, F.Cu at (185.4, 55.9)
- added TP1: TestPoint, proto_board:pad, F.Cu at (132.1, 45.7)
- added TP1: TestPoint, proto_board:pad, F.Cu at (111.8, 66.0)
- added TP1: TestPoint, proto_board:pad, F.Cu at (119.4, 76.2)
- added TP1: TestPoint, proto_board:pad, F.Cu at (99.1, 43.2)
- added TP1: TestPoint, proto_board:pad, F.Cu at (94.0, 45.7)
- added TP1: TestPoint, proto_board:pad, F.Cu at (144.8, 68.6)
- added TP1: TestPoint, proto_board:pad, F.Cu at (114.3, 50.8)
- added TP1: TestPoint, proto_board:pad, F.Cu at (94.0, 86.4)
- added TP1: TestPoint, proto_board:pad, F.Cu at (190.5, 50.8)
- added TP1: TestPoint, proto_board:pad, F.Cu at (193.0, 61.0)
- added TP1: TestPoint, proto_board:pad, F.Cu at (104.1, 53.3)
- added TP1: TestPoint, proto_board:pad, F.Cu at (195.6, 61.0)
- added TP1: TestPoint, proto_board:pad, F.Cu at (109.2, 73.7)
- added TP1: TestPoint, proto_board:pad, F.Cu at (127.0, 45.7)
- added TP1: TestPoint, proto_board:pad, F.Cu at (91.4, 96.5)
- added TP1: TestPoint, proto_board:pad, F.Cu at (142.2, 61.0)
- added TP1: TestPoint, proto_board:pad, F.Cu at (99.1, 78.7)
- added TP1: TestPoint, proto_board:pad, F.Cu at (91.4, 71.1)
- added TP1: TestPoint, proto_board:pad, F.Cu at (154.9, 55.9)
- added TP1: TestPoint, proto_board:pad, F.Cu at (180.3, 76.2)
- added TP1: TestPoint, proto_board:pad, F.Cu at (124.5, 61.0)
- added TP1: TestPoint, proto_board:pad, F.Cu at (139.7, 63.5)
- added TP1: TestPoint, proto_board:pad, F.Cu at (175.3, 48.3)
- added TP1: TestPoint, proto_board:pad, F.Cu at (180.3, 55.9)
- added TP1: TestPoint, proto_board:pad, F.Cu at (190.5, 86.4)
- added TP1: TestPoint, proto_board:pad, F.Cu at (195.6, 43.2)
- added TP1: TestPoint, proto_board:pad, F.Cu at (124.5, 73.7)
- added TP1: TestPoint, proto_board:pad, F.Cu at (91.4, 45.7)
- added TP1: TestPoint, proto_board:pad, F.Cu at (142.2, 71.1)
- added TP1: TestPoint, proto_board:pad, F.Cu at (106.7, 81.3)
- added TP1: TestPoint, proto_board:pad, F.Cu at (180.3, 68.6)
- added TP1: TestPoint, proto_board:pad, F.Cu at (198.1, 48.3)
- added TP1: TestPoint, proto_board:pad, F.Cu at (180.3, 78.7)
- added TP1: TestPoint, proto_board:pad, F.Cu at (170.2, 81.3)
- added TP1: TestPoint, proto_board:pad, F.Cu at (190.5, 63.5)
- added TP1: TestPoint, proto_board:pad, F.Cu at (99.1, 61.0)
- added TP1: TestPoint, proto_board:pad, F.Cu at (96.5, 71.1)
- added TP1: TestPoint, proto_board:pad, F.Cu at (121.9, 43.2)
- added TP1: TestPoint, proto_board:pad, F.Cu at (188.0, 58.4)
- added TP1: TestPoint, proto_board:pad, F.Cu at (167.6, 58.4)
- added TP1: TestPoint, proto_board:pad, F.Cu at (147.3, 76.2)
- added TP1: TestPoint, proto_board:pad, F.Cu at (116.8, 73.7)
- added TP1: TestPoint, proto_board:pad, F.Cu at (96.5, 91.4)
- added TP1: TestPoint, proto_board:pad, F.Cu at (109.2, 68.6)
- added TP1: TestPoint, proto_board:pad, F.Cu at (175.3, 94.0)
- added TP1: TestPoint, proto_board:pad, F.Cu at (154.9, 86.4)
- added TP1: TestPoint, proto_board:pad, F.Cu at (144.8, 61.0)
- added TP1: TestPoint, proto_board:pad, F.Cu at (134.6, 53.3)
- added TP1: TestPoint, proto_board:pad, F.Cu at (170.2, 63.5)
- added TP1: TestPoint, proto_board:pad, F.Cu at (167.6, 68.6)
- added TP1: TestPoint, proto_board:pad, F.Cu at (193.0, 76.2)
- added TP1: TestPoint, proto_board:pad, F.Cu at (114.3, 81.3)
- added TP1: TestPoint, proto_board:pad, F.Cu at (116.8, 45.7)
- added TP1: TestPoint, proto_board:pad, F.Cu at (165.1, 88.9)
- added TP1: TestPoint, proto_board:pad, F.Cu at (116.8, 81.3)
- added TP1: TestPoint, proto_board:pad, F.Cu at (134.6, 71.1)
- added TP1: TestPoint, proto_board:pad, F.Cu at (195.6, 76.2)
- added TP1: TestPoint, proto_board:pad, F.Cu at (99.1, 48.3)
- added TP1: TestPoint, proto_board:pad, F.Cu at (149.9, 71.1)
- added TP1: TestPoint, proto_board:pad, F.Cu at (175.3, 68.6)
- added TP1: TestPoint, proto_board:pad, F.Cu at (190.5, 45.7)
- added TP1: TestPoint, proto_board:pad, F.Cu at (114.3, 76.2)
- added TP1: TestPoint, proto_board:pad, F.Cu at (193.0, 88.9)
- added TP1: TestPoint, proto_board:pad, F.Cu at (157.5, 78.7)
- added TP1: TestPoint, proto_board:pad, F.Cu at (162.6, 43.2)
- added TP1: TestPoint, proto_board:pad, F.Cu at (94.0, 88.9)
- added TP1: TestPoint, proto_board:pad, F.Cu at (147.3, 81.3)
- added TP1: TestPoint, proto_board:pad, F.Cu at (111.8, 50.8)
- added TP1: TestPoint, proto_board:pad, F.Cu at (132.1, 61.0)
- added TP1: TestPoint, proto_board:pad, F.Cu at (116.8, 55.9)
- added TP1: TestPoint, proto_board:pad, F.Cu at (185.4, 58.4)
- added TP1: TestPoint, proto_board:pad, F.Cu at (144.8, 58.4)
- added TP1: TestPoint, proto_board:pad, F.Cu at (114.3, 68.6)
- added TP1: TestPoint, proto_board:pad, F.Cu at (193.0, 45.7)
- added TP1: TestPoint, proto_board:pad, F.Cu at (111.8, 58.4)
- added TP1: TestPoint, proto_board:pad, F.Cu at (154.9, 68.6)
- added TP1: TestPoint, proto_board:pad, F.Cu at (99.1, 71.1)
- added TP1: TestPoint, proto_board:pad, F.Cu at (185.4, 83.8)
- added TP1: TestPoint, proto_board:pad, F.Cu at (167.6, 48.3)
- added TP1: TestPoint, proto_board:pad, F.Cu at (114.3, 43.2)
- added TP1: TestPoint, proto_board:pad, F.Cu at (147.3, 66.0)
- added TP1: TestPoint, proto_board:pad, F.Cu at (106.7, 68.6)
- added TP1: TestPoint, proto_board:pad, F.Cu at (134.6, 61.0)
- added TP1: TestPoint, proto_board:pad, F.Cu at (144.8, 53.3)
- added TP1: TestPoint, proto_board:pad, F.Cu at (129.5, 43.2)
- added TP1: TestPoint, proto_board:pad, F.Cu at (170.2, 53.3)
- added TP1: TestPoint, proto_board:pad, F.Cu at (139.7, 73.7)
- added TP1: TestPoint, proto_board:pad, F.Cu at (172.7, 58.4)
- added TP1: TestPoint, proto_board:pad, F.Cu at (175.3, 63.5)
- added TP1: TestPoint, proto_board:pad, F.Cu at (195.6, 91.4)
- added TP1: TestPoint, proto_board:pad, F.Cu at (180.3, 48.3)
- added TP1: TestPoint, proto_board:pad, F.Cu at (106.7, 76.2)
- added TP1: TestPoint, proto_board:pad, F.Cu at (193.0, 83.8)
- added TP1: TestPoint, proto_board:pad, F.Cu at (91.4, 88.9)
- added TP1: TestPoint, proto_board:pad, F.Cu at (137.2, 76.2)
- added TP1: TestPoint, proto_board:pad, F.Cu at (132.1, 58.4)
- added TP1: TestPoint, proto_board:pad, F.Cu at (170.2, 45.7)
- added TP1: TestPoint, proto_board:pad, F.Cu at (167.6, 86.4)
- added TP1: TestPoint, proto_board:pad, F.Cu at (177.8, 94.0)
- added TP1: TestPoint, proto_board:pad, F.Cu at (104.1, 78.7)
- added TP1: TestPoint, proto_board:pad, F.Cu at (96.5, 66.0)
- added TP1: TestPoint, proto_board:pad, F.Cu at (94.0, 53.3)
- added TP1: TestPoint, proto_board:pad, F.Cu at (116.8, 53.3)
- added TP1: TestPoint, proto_board:pad, F.Cu at (149.9, 73.7)
- added TP1: TestPoint, proto_board:pad, F.Cu at (154.9, 61.0)
- added TP1: TestPoint, proto_board:pad, F.Cu at (119.4, 71.1)
- added TP1: TestPoint, proto_board:pad, F.Cu at (96.5, 43.2)
- added TP1: TestPoint, proto_board:pad, F.Cu at (109.2, 81.3)
- added TP1: TestPoint, proto_board:pad, F.Cu at (170.2, 48.3)
- added TP1: TestPoint, proto_board:pad, F.Cu at (165.1, 63.5)
- added TP1: TestPoint, proto_board:pad, F.Cu at (193.0, 78.7)
- added TP1: TestPoint, proto_board:pad, F.Cu at (188.0, 43.2)
- added TP1: TestPoint, proto_board:pad, F.Cu at (160.0, 45.7)
- added TP1: TestPoint, proto_board:pad, F.Cu at (165.1, 48.3)
- added TP1: TestPoint, proto_board:pad, F.Cu at (177.8, 63.5)
- added TP1: TestPoint, proto_board:pad, F.Cu at (182.9, 71.1)
- added TP1: TestPoint, proto_board:pad, F.Cu at (190.5, 61.0)
- added TP1: TestPoint, proto_board:pad, F.Cu at (109.2, 58.4)
- added TP1: TestPoint, proto_board:pad, F.Cu at (177.8, 81.3)
- added TP1: TestPoint, proto_board:pad, F.Cu at (175.3, 71.1)
- added TP1: TestPoint, proto_board:pad, F.Cu at (134.6, 78.7)
- added TP1: TestPoint, proto_board:pad, F.Cu at (167.6, 61.0)
- added TP1: TestPoint, proto_board:pad, F.Cu at (182.9, 68.6)
- added TP1: TestPoint, proto_board:pad, F.Cu at (157.5, 81.3)
- added TP1: TestPoint, proto_board:pad, F.Cu at (96.5, 45.7)
- added TP1: TestPoint, proto_board:pad, F.Cu at (160.0, 50.8)
- added TP1: TestPoint, proto_board:pad, F.Cu at (152.4, 66.0)
- added TP1: TestPoint, proto_board:pad, F.Cu at (127.0, 66.0)
- added TP1: TestPoint, proto_board:pad, F.Cu at (142.2, 63.5)
- added TP1: TestPoint, proto_board:pad, F.Cu at (190.5, 83.8)
- added TP1: TestPoint, proto_board:pad, F.Cu at (177.8, 53.3)
- added TP1: TestPoint, proto_board:pad, F.Cu at (152.4, 61.0)
- added TP1: TestPoint, proto_board:pad, F.Cu at (188.0, 78.7)
- added TP1: TestPoint, proto_board:pad, F.Cu at (106.7, 71.1)
- added TP1: TestPoint, proto_board:pad, F.Cu at (111.8, 53.3)
- added TP1: TestPoint, proto_board:pad, F.Cu at (162.6, 88.9)
- added TP1: TestPoint, proto_board:pad, F.Cu at (106.7, 48.3)
- added TP1: TestPoint, proto_board:pad, F.Cu at (152.4, 58.4)
- added TP1: TestPoint, proto_board:pad, F.Cu at (142.2, 66.0)
- added TP1: TestPoint, proto_board:pad, F.Cu at (177.8, 66.0)
- added TP1: TestPoint, proto_board:pad, F.Cu at (195.6, 50.8)
- added TP1: TestPoint, proto_board:pad, F.Cu at (162.6, 73.7)
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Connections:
- J1 pad A1: (no net) -> /A1
- J1 pad A10: (no net) -> unconnected-(J1-Pin_a10-PadA10)
- J1 pad A11: (no net) -> unconnected-(J1-Pin_A11-PadA11)
- J1 pad A12: (no net) -> unconnected-(J1-Pin_a12-PadA12)
- J1 pad A13: (no net) -> unconnected-(J1-Pin_a13-PadA13)
- J1 pad A14: (no net) -> unconnected-(J1-Pin_a14-PadA14)
- J1 pad A15: (no net) -> unconnected-(J1-Pin_a15-PadA15)
- J1 pad A16: (no net) -> unconnected-(J1-Pin_a16-PadA16)
- J1 pad A17: (no net) -> unconnected-(J1-Pin_a17-PadA17)
- J1 pad A18: (no net) -> unconnected-(J1-Pin_a18-PadA18)
- J1 pad A19: (no net) -> unconnected-(J1-Pin_a19-PadA19)
- J1 pad A2: (no net) -> /A2
- J1 pad A20: (no net) -> unconnected-(J1-Pin_a20-PadA20)
- J1 pad A21: (no net) -> unconnected-(J1-Pin_a21-PadA21)
- J1 pad A22: (no net) -> unconnected-(J1-Pin_a22-PadA22)
- J1 pad A23: (no net) -> unconnected-(J1-Pin_a23-PadA23)
- J1 pad A24: (no net) -> unconnected-(J1-Pin_a24-PadA24)
- J1 pad A25: (no net) -> unconnected-(J1-Pin_a25-PadA25)
- J1 pad A26: (no net) -> unconnected-(J1-Pin_a26-PadA26)
- J1 pad A27: (no net) -> unconnected-(J1-Pin_a27-PadA27)
- J1 pad A28: (no net) -> unconnected-(J1-Pin_a28-PadA28)
- J1 pad A29: (no net) -> unconnected-(J1-Pin_a29-PadA29)
- J1 pad A3: (no net) -> /A3
- J1 pad A30: (no net) -> unconnected-(J1-Pin_a30-PadA30)
- J1 pad A31: (no net) -> unconnected-(J1-Pin_a31-PadA31)
- J1 pad A32: (no net) -> unconnected-(J1-Pin_a32-PadA32)
- J1 pad A33: (no net) -> unconnected-(J1-Pin_a33-PadA33)
- J1 pad A34: (no net) -> unconnected-(J1-Pin_a34-PadA34)
- J1 pad A35: (no net) -> unconnected-(J1-Pin_a35-PadA35)
- J1 pad A36: (no net) -> unconnected-(J1-Pin_a36-PadA36)
- J1 pad A37: (no net) -> unconnected-(J1-Pin_a37-PadA37)
- J1 pad A38: (no net) -> unconnected-(J1-Pin_a38-PadA38)
- J1 pad A39: (no net) -> unconnected-(J1-Pin_a39-PadA39)
- J1 pad A4: (no net) -> /A4
- J1 pad A40: (no net) -> unconnected-(J1-Pin_a40-PadA40)
- J1 pad A41: (no net) -> unconnected-(J1-Pin_a41-PadA41)
- J1 pad A42: (no net) -> unconnected-(J1-Pin_a42-PadA42)
- J1 pad A43: (no net) -> unconnected-(J1-Pin_a43-PadA43)
- J1 pad A44: (no net) -> unconnected-(J1-Pin_a44-PadA44)
- J1 pad A45: (no net) -> unconnected-(J1-Pin_a45-PadA45)
- J1 pad A46: (no net) -> unconnected-(J1-Pin_a46-PadA46)
- J1 pad A47: (no net) -> unconnected-(J1-Pin_a47-PadA47)
- J1 pad A48: (no net) -> unconnected-(J1-Pin_a48-PadA48)
- J1 pad A49: (no net) -> unconnected-(J1-Pin_a49-PadA49)
- J1 pad A5: (no net) -> unconnected-(J1-Pin_a5-PadA5)
- J1 pad A6: (no net) -> unconnected-(J1-Pin_a6-PadA6)
- J1 pad A7: (no net) -> unconnected-(J1-Pin_a7-PadA7)
- J1 pad A8: (no net) -> unconnected-(J1-Pin_a8-PadA8)
- J1 pad A9: (no net) -> unconnected-(J1-Pin_a9-PadA9)
- J1 pad B1: (no net) -> /B1
- J1 pad B10: (no net) -> unconnected-(J1-Pin_b10-PadB10)
- J1 pad B11: (no net) -> unconnected-(J1-Pin_b11-PadB11)
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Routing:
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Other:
- board size 80 x 50 mm -> 113.1 x 62.3 mm
- board text added: "Conn_02x25_Odd_Even"
